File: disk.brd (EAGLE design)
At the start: 40 x 40 mm, 0 parts

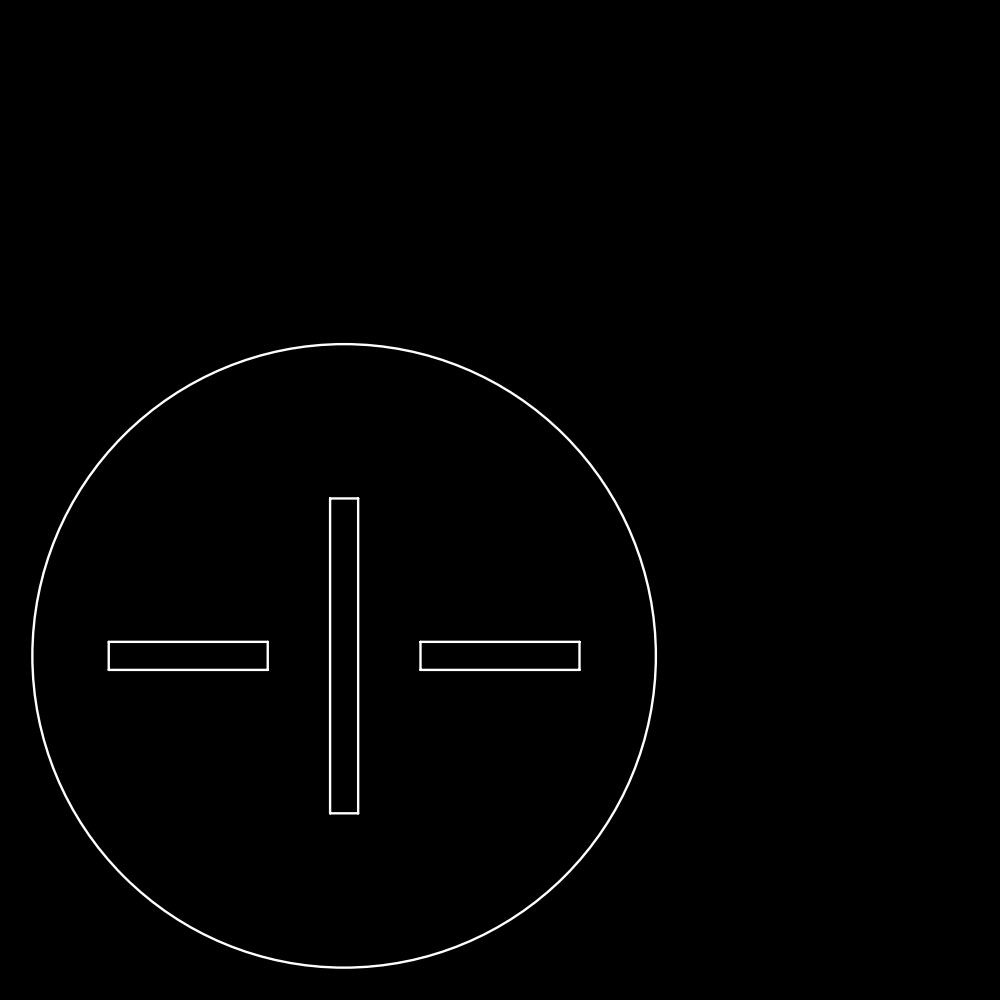
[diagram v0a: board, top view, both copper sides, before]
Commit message: reworked boards and gerber files
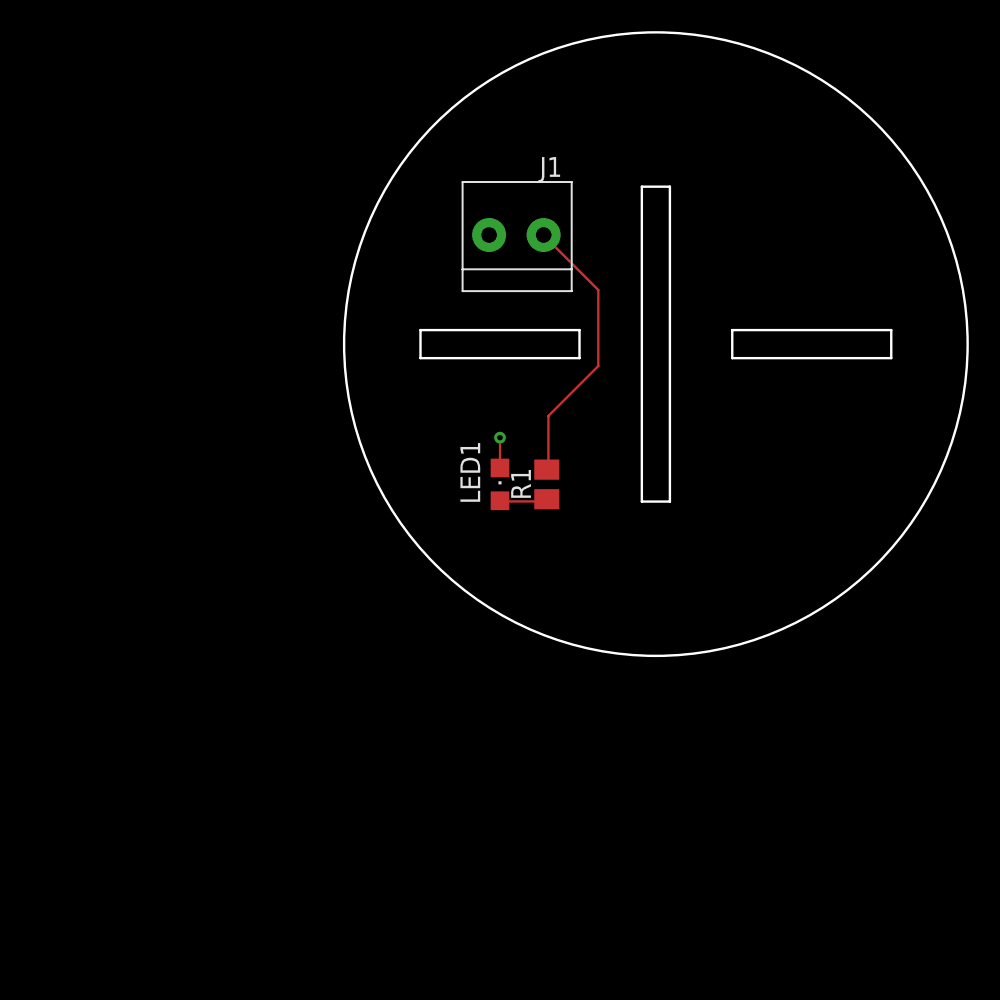
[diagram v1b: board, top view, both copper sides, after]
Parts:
- added J1: 1X2-3.5MM, adafruit:1X2-3.5MM
- added LED1: (no value), adafruit:CHIPLED_0805
- added R1: (no value), adafruit:M0805
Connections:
- new net GND: J1.2, LED1.C
- new net N$1: J1.1, R1.2
- new net N$2: LED1.A, R1.1
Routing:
- net N$1: track 0.00 -> 17.9 mm
- net N$2: track 0.00 -> 3.12 mm
- net GND: track 0.00 -> 2.12 mm, vias 0 -> 1
- added copper zone on layer 16, net GND
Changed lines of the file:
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@@
 <layer number="45" name="Holes" color="7" fill="1" visible="yes" active="yes"/>
 <layer number="46" name="Milling" color="3" fill="1" visible="no" active="yes"/>
-<layer number="47" name="Measures" color="7" fill="1" visible="no" active="yes"/>
+<layer number="47" name="Measures" color="7" fill="1" visible="yes" active="yes"/>
 <layer number="48" name="Document" color="7" fill="1" visible="yes" active="yes"/>
 <layer number="49" name="Reference" color="7" fill="1" visible="yes" active="yes"/>
@@
 <board>
 <plain>
-<circle x="0" y="0" radius="20" width="0.1524" layer="20"/>
-<wire x1="-0.9" y1="10.1" x2="-0.9" y2="-10.1" width="0.1524" layer="20"/>
-<wire x1="-0.9" y1="-10.1" x2="0.9" y2="-10.1" width="0.1524" layer="20"/>
-<wire x1="0.9" y1="-10.1" x2="0.9" y2="10.1" width="0.1524" layer="20"/>
-<wire x1="0.9" y1="10.1" x2="-0.9" y2="10.1" width="0.1524" layer="20"/>
-<wire x1="4.9" y1="0.9" x2="4.9" y2="-0.9" width="0.1524" layer="20"/>
-<wire x1="4.9" y1="-0.9" x2="15.1" y2="-0.9" width="0.1524" layer="20"/>
-<wire x1="15.1" y1="-0.9" x2="15.1" y2="0.9" width="0.1524" layer="20"/>
-<wire x1="4.9" y1="0.9" x2="15.1" y2="0.9" width="0.1524" layer="20"/>
-<wire x1="-15.1" y1="0.9" x2="-4.9" y2="0.9" width="0.1524" layer="20"/>
-<wire x1="-4.9" y1="0.9" x2="-4.9" y2="-0.9" width="0.1524" layer="20"/>
-<wire x1="-4.9" y1="-0.9" x2="-15.1" y2="-0.9" width="0.1524" layer="20"/>
-<wire x1="-15.1" y1="-0.9" x2="-15.1" y2="0.9" width="0.1524" layer="20"/>
-<dimension x1="-15" y1="-0.9" x2="-15" y2="0.9" x3="-21" y3="0" textsize="1.778" layer="20"/>
-<dimension x1="15" y1="-0.9" x2="15" y2="0.9" x3="21" y3="0" textsize="1.778" layer="20"/>
-<dimension x1="-4.9" y1="-0.9" x2="-15.1" y2="-0.9" x3="-10" y3="-4" textsize="1.778" layer="20"/>
-<dimension x1="4.9" y1="-0.9" x2="15.1" y2="-0.9" x3="10" y3="-4" textsize="1.778" layer="20"/>
-<dimension x1="0.9" y1="-10.1" x2="0.9" y2="10.1" x3="-2" y3="0" textsize="1.778" layer="20"/>
-<dimension x1="0.9" y1="10.1" x2="-0.9" y2="10.1" x3="0" y3="11" textsize="1.778" layer="20"/>
-<dimension x1="0" y1="0" x2="4.9" y2="0" x3="2.45" y3="-12" textsize="1.778" layer="20"/>
-<dimension x1="15.1" y1="0" x2="20" y2="0" x3="17.55" y3="-9" textsize="1.778" layer="20"/>
-<dimension x1="0" y1="0" x2="16" y2="12" x3="8" y3="6" textsize="1.778" layer="20"/>
+<circle x="20" y="20" radius="20" width="0.1524" layer="20"/>
+<wire x1="19.1" y1="30.1" x2="19.1" y2="9.9" width="0.1524" layer="20"/>
+<wire x1="19.1" y1="9.9" x2="20.9" y2="9.9" width="0.1524" layer="20"/>
+<wire x1="20.9" y1="9.9" x2="20.9" y2="30.1" width="0.1524" layer="20"/>
+<wire x1="20.9" y1="30.1" x2="19.1" y2="30.1" width="0.1524" layer="20"/>
+<wire x1="24.9" y1="20.9" x2="24.9" y2="19.1" width="0.1524" layer="20"/>
+<wire x1="24.9" y1="19.1" x2="35.1" y2="19.1" width="0.1524" layer="20"/>
+<wire x1="35.1" y1="19.1" x2="35.1" y2="20.9" width="0.1524" layer="20"/>
+<wire x1="24.9" y1="20.9" x2="35.1" y2="20.9" width="0.1524" layer="20"/>
+<wire x1="4.9" y1="20.9" x2="15.1" y2="20.9" width="0.1524" layer="20"/>
+<wire x1="15.1" y1="20.9" x2="15.1" y2="19.1" width="0.1524" layer="20"/>
+<wire x1="15.1" y1="19.1" x2="4.9" y2="19.1" width="0.1524" layer="20"/>
+<wire x1="4.9" y1="19.1" x2="4.9" y2="20.9" width="0.1524" layer="20"/>
+<dimension x1="5" y1="19.1" x2="5" y2="20.9" x3="-1" y3="20" textsize="1.778" layer="47"/>
+<dimension x1="35" y1="19.1" x2="35" y2="20.9" x3="41" y3="20" textsize="1.778" layer="47"/>
+<dimension x1="15.1" y1="19.1" x2="4.9" y2="19.1" x3="10" y3="16" textsize="1.778" layer="47"/>
+<dimension x1="24.9" y1="19.1" x2="35.1" y2="19.1" x3="30" y3="16" textsize="1.778" layer="47"/>
+<dimension x1="20.9" y1="9.9" x2="20.9" y2="30.1" x3="18" y3="20" textsize="1.778" layer="47"/>
+<dimension x1="20.9" y1="30.1" x2="19.1" y2="30.1" x3="20" y3="31" textsize="1.778" layer="47"/>
+<dimension x1="20" y1="20" x2="24.9" y2="20" x3="22.45" y3="8" textsize="1.778" layer="47"/>
+<dimension x1="35.1" y1="20" x2="40" y2="20" x3="37.55" y3="11" textsize="1.778" layer="47"/>
+<dimension x1="20" y1="20" x2="36" y2="32" x3="28" y3="26" textsize="1.778" layer="47"/>
 </plain>
 <attributes>
@@
 <autorouter>
 <pass name="Default">
-<param name="RoutingGrid" value="50mil"/>
+<param name="RoutingGrid" value="6mil"/>
 <param name="AutoGrid" value="1"/>
 <param name="Efforts" value="0"/>
 <param name="TopRouterVariant" value="1"/>
 <param name="tpViaShape" value="round"/>
-<param name="PrefDir.1" value="a"/>
+<param name="PrefDir.1" value="*"/>
 <param name="PrefDir.2" value="0"/>
 <param name="PrefDir.3" value="0"/>
@@
 <param name="PrefDir.14" value="0"/>
 <param name="PrefDir.15" value="0"/>
-<param name="PrefDir.16" value="a"/>
-<param name="cfVia" value="8"/>
+<param name="PrefDir.16" value="*"/>
+<param name="cfVia" value="90"/>
 <param name="cfNonPref" value="5"/>
 <param name="cfChangeDir" value="2"/>
@@
 </pass>
 <pass name="Follow-me" refer="Default" active="yes">
+<param name="cfVia" value="8"/>
 </pass>
 <pass name="Busses" refer="Default" active="yes">
+<param name="cfVia" value="8"/>
 <param name="cfNonPref" value="4"/>
 <param name="cfBusImpact" value="4"/>
@@
 <pass name="Optimize1" refer="Default" active="yes">
 <param name="cfVia" value="99"/>
-<param name="cfExtdStep" value="10"/>
-<param name="cfHugging" value="1"/>
-<param name="mnExtdSteps" value="1"/>
-<param name="mnRipupLevel" value="0"/>
 </pass>
 <pass name="Optimize2" refer="Optimize1" active="yes">
-<param name="cfNonPref" value="0"/>
-<param name="cfChangeDir" value="6"/>
-<param name="cfExtdStep" value="0"/>
-<param name="cfBonusStep" value="2"/>
-<param name="cfMalusStep" value="2"/>
-<param name="cfPadImpact" value="2"/>
-<param name="cfSmdImpact" value="2"/>
-<param name="cfHugging" value="0"/>
 </pass>
 <pass name="Optimize3" refer="Optimize2" active="yes">
-<param name="cfChangeDir" value="8"/>
+<param name="cfBonusStep" value="0"/>
+<param name="cfMalusStep" value="0"/>
 <param name="cfPadImpact" value="0"/>
 <param name="cfSmdImpact" value="0"/>
+<param name="cfHugging" value="0"/>
 </pass>
 <pass name="Optimize4" refer="Optimize3" active="yes">
-<param name="cfChangeDir" value="25"/>
 </pass>
 </autorouter>
 <elements>
+<element name="J1" library="adafruit" library_urn="urn:adsk.eagle:library:420" package="1X2-3.5MM" package3d_urn="urn:adsk.eagle:package:6240635/1" value="1X2-3.5MM" x="11" y="27" smashed="yes">
+<attribute name="NAME" x="14" y="32" size="1.27" layer="25" rot="R180"/>
+</element>
+<element name="R1" library="adafruit" library_urn="urn:adsk.eagle:library:420" package="M0805" package3d_urn="urn:adsk.eagle:package:6240587/1" value="" x="13" y="11" smashed="yes" rot="R90">
+<attribute name="NAME" x="11.984" y="9.984" size="1.27" layer="25" rot="R90"/>
+<attribute name="VALUE" x="15.286" y="9.984" size="1.27" layer="27" rot="R90"/>
+</element>
+<element name="LED1" library="adafruit" library_urn="urn:adsk.eagle:library:420" package="CHIPLED_0805" package3d_urn="urn:adsk.eagle:package:6240559/1" value="" x="10" y="11" smashed="yes">
+<attribute name="NAME" x="8.73" y="9.73" size="1.27" layer="25" rot="R90"/>
+<attribute name="VALUE" x="12.54" y="9.73" size="1.27" layer="27" rot="R90"/>
+</element>
 </elements>
 <signals>
+<signal name="N$1">
+<contactref element="J1" pad="1"/>
+<contactref element="R1" pad="2"/>
+<wire x1="13.1064" y1="15.3924" x2="13.1064" y2="12.0396" width="0.1524" layer="1"/>
+<wire x1="16.3068" y1="18.5928" x2="13.1064" y2="15.3924" width="0.1524" layer="1"/>
+<wire x1="16.3068" y1="23.4696" x2="16.3068" y2="18.5928" width="0.1524" layer="1"/>
+<wire x1="12.8016" y1="26.9748" x2="16.3068" y2="23.4696" width="0.1524" layer="1"/>
+<wire x1="13.1064" y1="12.0396" x2="13" y2="11.95" width="0.1524" layer="1"/>
+<wire x1="12.8016" y1="26.9748" x2="12.8" y2="27" width="0.1524" layer="1"/>
+</signal>
+<signal name="N$2">
+<contactref element="R1" pad="1"/>
+<contactref element="LED1" pad="A"/>
+<wire x1="12.954" y1="9.906" x2="10.0584" y2="9.906" width="0.1524" layer="1"/>
+<wire x1="10.0584" y1="9.906" x2="10" y2="9.95" width="0.1524" layer="1"/>
+<wire x1="12.954" y1="9.906" x2="13" y2="10.05" width="0.1524" layer="1"/>
+</signal>
+<signal name="GND">
+<contactref element="LED1" pad="C"/>
+<contactref element="J1" pad="2"/>
+<polygon width="0.1524" layer="16">
+<vertex x="40" y="20" curve="180"/>
+<vertex x="0" y="20" curve="180"/>
+</polygon>
+<wire x1="9.906" y1="12.192" x2="10" y2="12.05" width="0.1524" layer="1"/>
+<via x="10" y="14" extent="1-16" drill="0.35"/>
+<wire x1="10" y1="12.05" x2="10" y2="14" width="0.1524" layer="1"/>
+</signal>
 </signals>
 <mfgpreviewcolors>
@@
 </board>
 </drawing>
+<compatibility>
+<note version="8.2" severity="warning">
+Since Version 8.2, EAGLE supports online libraries. The ids
+of those online libraries will not be understood (or retained)
+with this version.
+</note>
+<note version="8.3" severity="warning">
+Since Version 8.3, EAGLE supports URNs for individual library
+assets (packages, symbols, and devices). The URNs of those assets
+will not be understood (or retained) with this version.
+</note>
+<note version="8.3" severity="warning">
+Since Version 8.3, EAGLE supports the association of 3D packages
+with devices in libraries, schematics, and board files. Those 3D
+packages will not be understood (or retained) with this version.
+</note>
+</compatibility>
 </eagle>
